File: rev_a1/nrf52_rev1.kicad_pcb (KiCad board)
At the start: 2 copper layers, 25.4 x 48.3 mm, 27 parts, among them P1 CONN_01X18, P2 CONN_01X18, P3 USB_OTG, U1 nRF52832, U2 CP2102, U3 LT1129CST-3.3, Y1 32K, Y2 32M

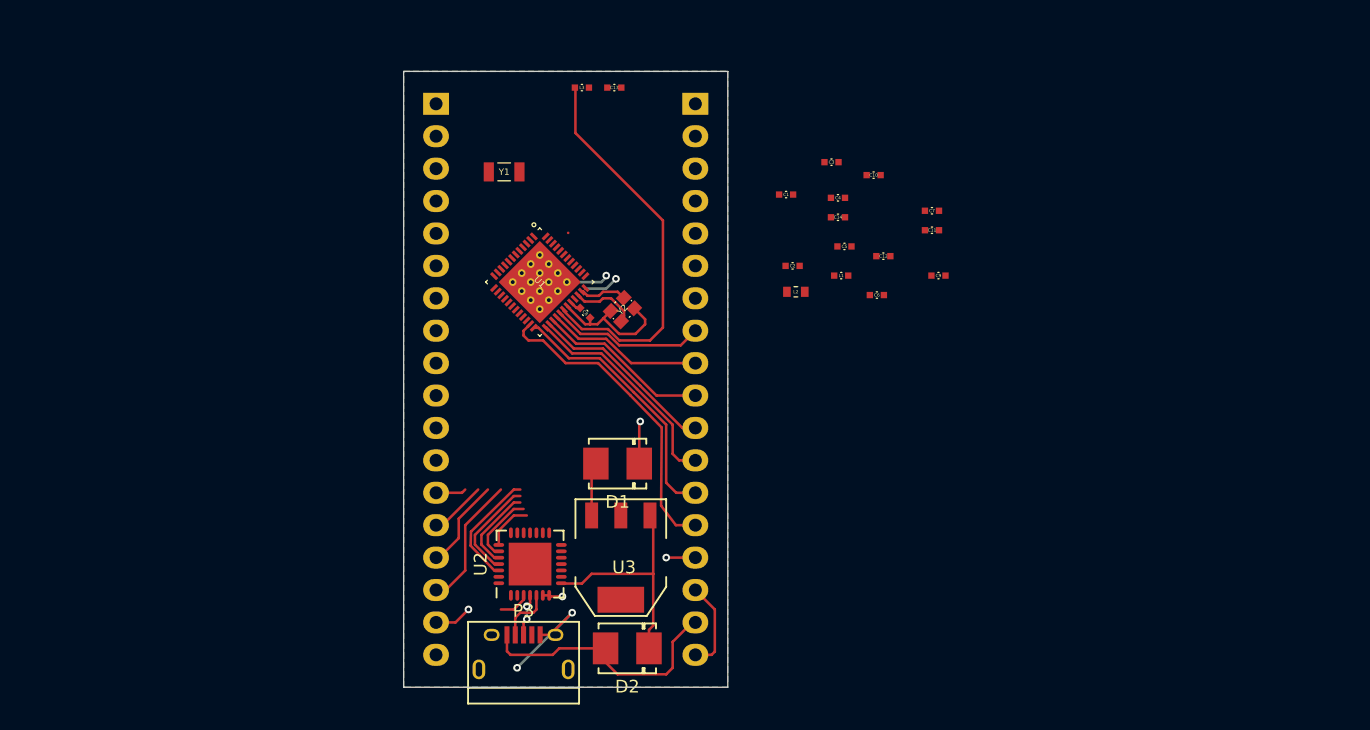
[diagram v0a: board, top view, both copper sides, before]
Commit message: WIP
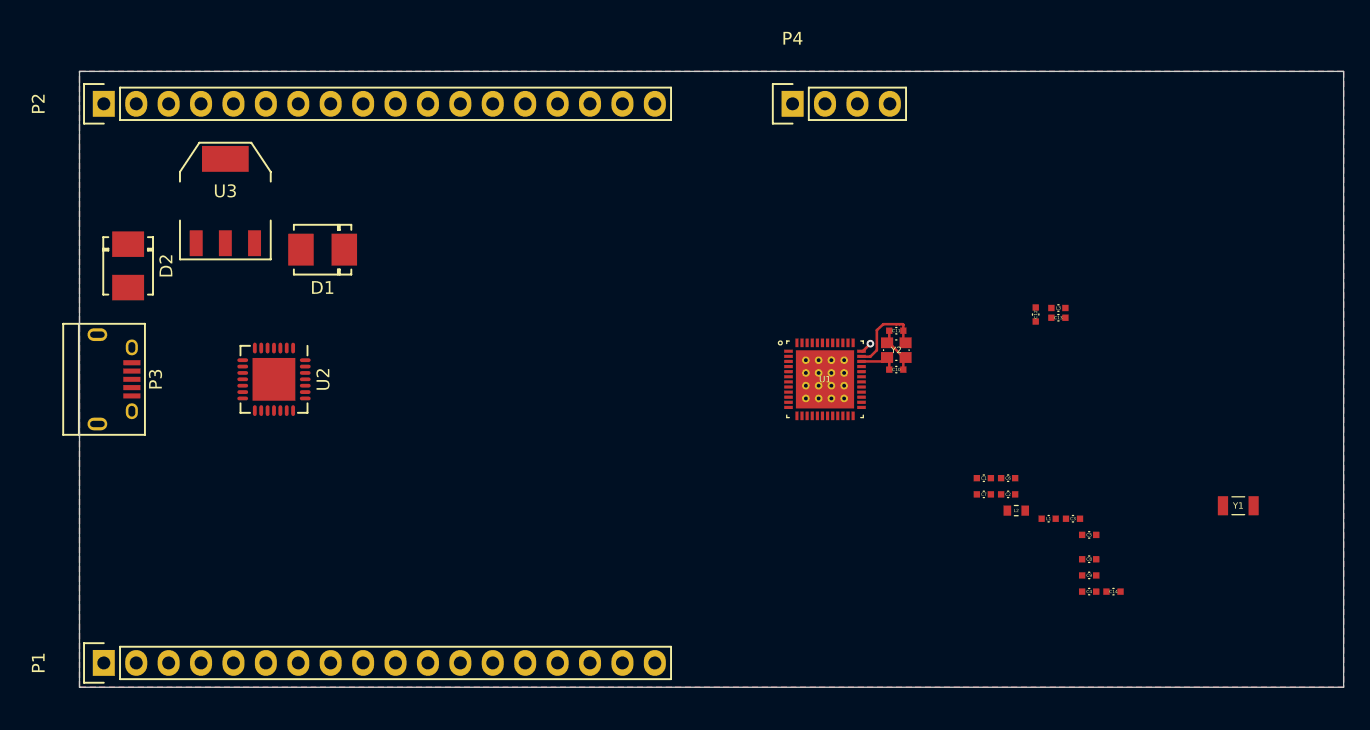
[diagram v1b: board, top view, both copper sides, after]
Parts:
- added P4: I2C_OLED, Socket_Strips:Socket_Strip_Straight_1x04, F.Cu at (81.3, 27.9)
- P1, P2: moved to F.Cu
- moved Y1 63.2 mm to (116.2, 59.4), turned to 0 degrees
- moved P1 51.0 mm to (27.3, 71.8), turned to 90 degrees
- moved D2 49.3 mm to (29.2, 40.6), turned to 270 degrees
- moved P2 46.4 mm to (27.3, 27.9), turned to 90 degrees
- moved C8 44.0 mm to (104.5, 63.6), turned to 0 degrees
- moved U3 41.7 mm to (36.8, 35.6), turned to 0 degrees
- moved L3 41.1 mm to (102.1, 43.9)
- moved C13 39.2 mm to (102.1, 44.7), turned to 180 degrees
- moved P3 38.8 mm to (27.9, 49.5), turned to 270 degrees
- moved C4 36.6 mm to (104.5, 66.2)
- moved C14 36.4 mm to (106.4, 66.2)
- moved C3 33.7 mm to (103.3, 60.5)
- moved C5 29.6 mm to (104.5, 61.7)
- moved D1 28.6 mm to (44.5, 39.4)
- moved C1 27.1 mm to (96.3, 57.3)
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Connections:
- net 3V3 renamed +3V3
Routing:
- net GND: track 57.1 -> 3.97 mm, vias 3 -> 0
- net Net-(C12-Pad1): track 30.9 -> 0.00 mm
- net P0.20: track 24.5 -> 0.00 mm
- net 5V_IN: track 20.7 -> 0.00 mm
- net P0.21: track 20.7 -> 0.00 mm
- net +5V: track 19.1 -> 0.00 mm
- net SWDCLK: track 17.4 -> 0.00 mm
- net SWDIO: track 14.8 -> 0.00 mm
- net P0.22: track 13.6 -> 0.00 mm
- net P0.23: track 12.4 -> 0.00 mm
- net P0.24: track 12.1 -> 0.00 mm
- net P0.19: track 10.4 -> 0.00 mm
- net P0.08: track 9.35 -> 0.00 mm
- net +3V3: track 10.2 -> 1.58 mm, vias 4 -> 1
- net P0.06: track 8.08 -> 0.00 mm
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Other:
- board size 25.4 x 48.3 mm -> 99.1 x 48.3 mm
